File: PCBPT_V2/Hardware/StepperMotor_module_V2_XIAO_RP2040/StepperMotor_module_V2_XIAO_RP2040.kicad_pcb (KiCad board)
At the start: 2 copper layers, 43 x 43 mm, 32 parts, among them IC1 ICM-20649, J1 1660, J2 battery, J3 External Ctrl, J4 Conn_01x03_Pin, J5 SW, U1 MOUDLE-SEEEDUINO-XIAO, U2 MCP73831-2-OT, U3 AP2112K-3.3

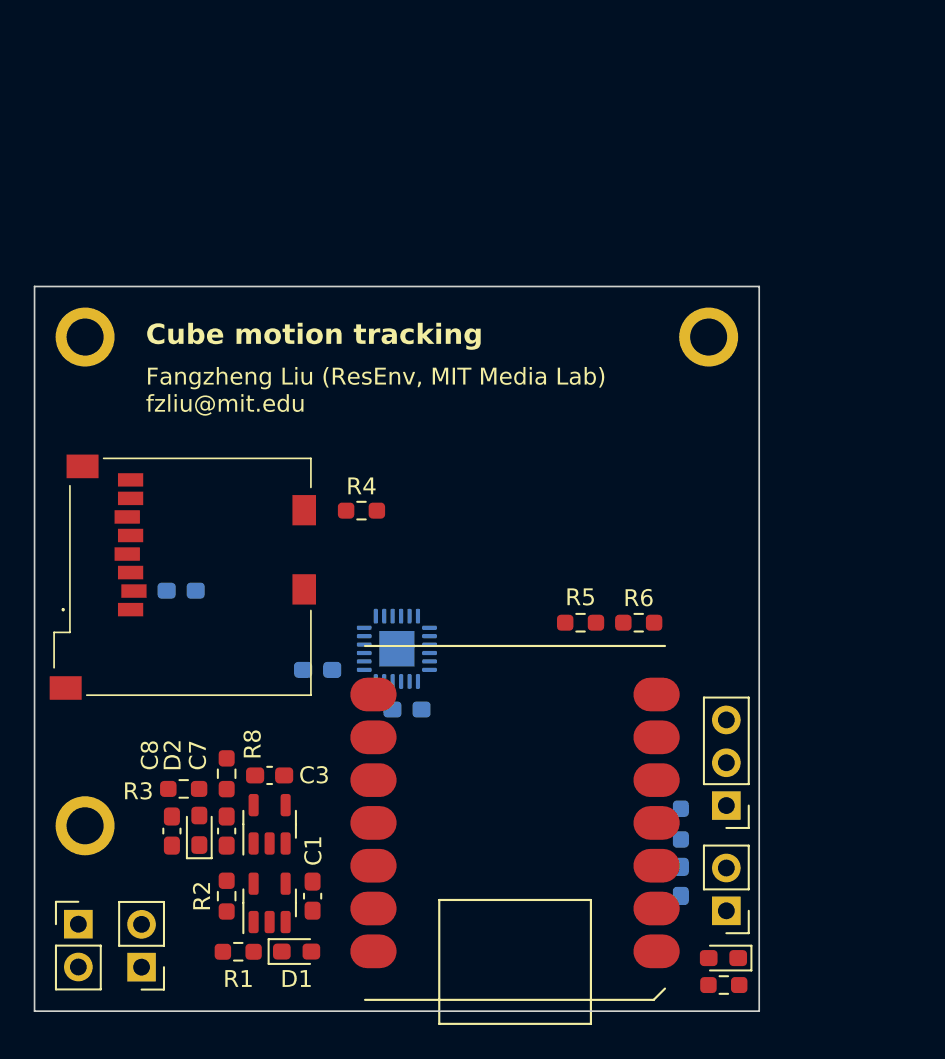
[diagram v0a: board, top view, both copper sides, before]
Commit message: udated by FZ
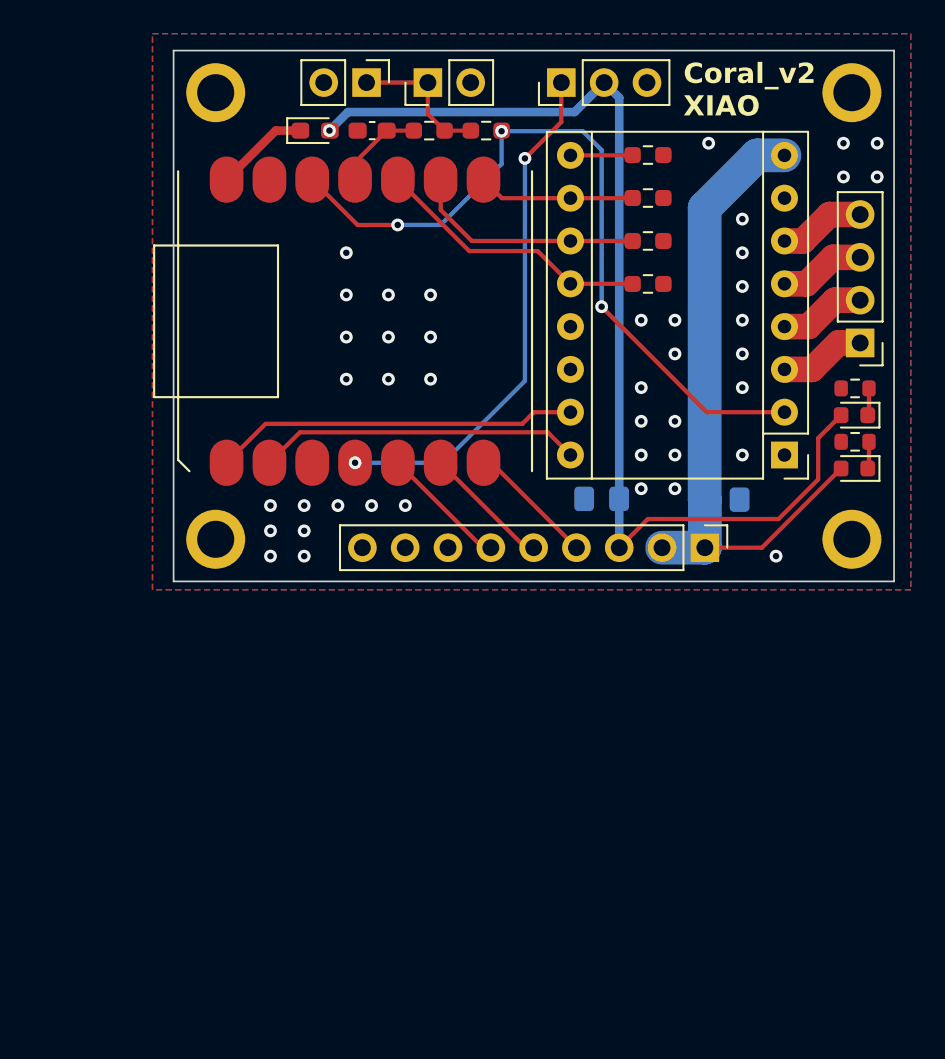
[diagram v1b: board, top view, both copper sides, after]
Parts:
- removed C4, C5, C6, C7: 0.1uF, Capacitor_SMD:C_0603_1608Metric_Pad1.08x0.95mm_HandSolder
- removed C8: 10uF, Capacitor_SMD:C_0603_1608Metric_Pad1.08x0.95mm_HandSolder
- removed C9: 0.01uF, Capacitor_SMD:C_0603_1608Metric_Pad1.08x0.95mm_HandSolder
- removed D3: Red, LED_SMD:LED_0603_1608Metric_Pad1.05x0.95mm_HandSolder
- removed IC1: ICM-20649, Package_DFN_QFN:HVQFN-24-1EP_4x4mm_P0.5mm_EP2.1x2.1mm
- removed J1: 1660, SamacSys_Parts:1660
- removed J2: battery, Connector_PinHeader_2.54mm:PinHeader_1x02_P2.54mm_Vertical
- removed R5, R6: 499K, Resistor_SMD:R_0603_1608Metric_Pad0.98x0.95mm_HandSolder
- removed R7, R9: 10K, Resistor_SMD:R_0603_1608Metric_Pad0.98x0.95mm_HandSolder
- removed U2: MCP73831-2-OT, Package_TO_SOT_SMD:SOT-23-5
- removed U3: AP2112K-3.3, Package_TO_SOT_SMD:SOT-23-5
- added A1: Pololu_Breakout_A4988, Module:Pololu_Breakout-16_15.2x20.3mm, F.Cu at (158.5, 82.0)
- added C2: 0.01uF, Capacitor_SMD:C_0603_1608Metric_Pad1.08x0.95mm_HandSolder, F.Cu at (134.0, 62.8)
- added D4: LED_Small_Filled, LED_SMD:LED_0603_1608Metric, F.Cu at (162.7, 82.8)
- added H4: M2, MountingHole:MountingHole_2.2mm_M2_ISO7380_Pad, F.Cu at (162.5, 60.5)
- added J6: Limit Switch, Connector_PinHeader_2.54mm:PinHeader_1x02_P2.54mm_Vertical, F.Cu at (133.7, 59.9)
- added J7: Limit Switch, Connector_PinHeader_2.54mm:PinHeader_1x02_P2.54mm_Vertical, F.Cu at (137.3, 59.9)
- added R10: 10k, Resistor_SMD:R_0603_1608Metric, F.Cu at (162.7, 81.2)
- added R11: 10K, Resistor_SMD:R_0603_1608Metric_Pad0.98x0.95mm_HandSolder, F.Cu at (140.8, 62.8)
- added R12: 100, Resistor_SMD:R_0603_1608Metric_Pad0.98x0.95mm_HandSolder, F.Cu at (137.4, 62.8)
- C1: footprint Capacitor_SMD:C_0603_1608Metric_Pad1.08x0.95mm_HandSolder -> Capacitor_SMD:C_0805_2012Metric_Pad1.18x1.45mm_HandSolder; moved to B.Cu
- C3: value 10uF -> 0.1uF; footprint Capacitor_SMD:C_0603_1608Metric_Pad1.08x0.95mm_HandSolder -> Capacitor_SMD:C_0805_2012Metric_Pad1.18x1.45mm_HandSolder; moved to B.Cu
- D1: value CHG -> LED_Small_Filled; footprint LED_SMD:LED_0603_1608Metric_Pad1.05x0.95mm_HandSolder -> LED_SMD:LED_0603_1608Metric
- J3: value External Ctrl -> Servo; footprint Connector_PinHeader_2.54mm:PinHeader_1x02_P2.54mm_Vertical -> Connector_PinHeader_2.54mm:PinHeader_1x03_P2.54mm_Vertical
- J4: value Conn_01x03_Pin -> Limit Switch; footprint Connector_PinHeader_2.54mm:PinHeader_1x03_P2.54mm_Vertical -> Connector_PinHeader_2.54mm:PinHeader_1x04_P2.54mm_Vertical
- J5: value SW -> Conn_01x09_Pin; footprint Connector_PinHeader_2.54mm:PinHeader_1x02_P2.54mm_Vertical -> Connector_PinHeader_2.54mm:PinHeader_1x09_P2.54mm_Vertical
- R1: value 1K -> 499K
- R2: value 1K -> 10K
- R3: value 1M -> 10K
- R4: value NC -> 10K
- R8: value 1M -> 10k; footprint Resistor_SMD:R_0603_1608Metric_Pad0.98x0.95mm_HandSolder -> Resistor_SMD:R_0603_1608Metric
- moved R1 53.2 mm to (150.4, 64.2)
- moved J3 50.1 mm to (145.3, 59.9), turned to 90 degrees
- moved R2 48.4 mm to (150.4, 66.8), turned to 0 degrees
- moved D1 45.9 mm to (162.7, 79.6), turned to 180 degrees
- moved R8 43.7 mm to (162.7, 78.0), turned to 180 degrees
- moved R3 42.6 mm to (150.4, 69.3)
- moved D2 42.1 mm to (130.7, 62.8), turned to 0 degrees
- moved J5 41.7 mm to (153.8, 87.5), turned to -90 degrees
- moved C1 33.8 mm to (154.8, 84.7), turned to 0 degrees
- moved J4 28.6 mm to (163.0, 75.3)
- moved C3 25.6 mm to (147.7, 84.6), turned to 180 degrees
- moved R4 21.7 mm to (150.4, 71.8)
- moved H1 18.7 mm to (124.8, 87.0)
- moved H2 16.4 mm to (124.8, 60.5)
- moved H3 14.7 mm to (162.5, 87.0)
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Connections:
- C1 pad 1: VBUS -> VPP
- C3 pad 1: +3V3 -> VCC
- D1 pad 2: VBUS -> VCC
- D2 pad 1: VBUS -> Net-(D2-K)
- D2 pad 2: +BATT -> VCC
- J3 pad 1: GND -> PWM_S
- J3 pad 2: /MCU-XIAO RP2040/EX_SIG -> VCC
- J4 pad 1: Net-(J4-Pin_1) -> 1B
- J4 pad 2: Net-(J4-Pin_2) -> 1A
- J4 pad 3: Net-(J4-Pin_3) -> 2A
- J5 pad 1: Net-(J2-Pin_2) -> VPP
- J5 pad 2: +BATT -> VPP
- R1 pad 1: Net-(D1-K) -> /A4988_Module/M_EN
- R1 pad 2: Net-(U2-STAT) -> GND
- R2 pad 1: Net-(U2-PROG) -> MS1
- R3 pad 1: GND -> MS2
- R3 pad 2: +BATT -> GND
- R4 pad 1: Net-(J1-CARD_DETECT_1) -> MS3
- R4 pad 2: +3V3 -> GND
- R8 pad 1: GND -> Net-(D1-K)
- R8 pad 2: +3V3 -> GND
- U1 pad 1: /MCU-XIAO RP2040/VBAT -> STEP
- U1 pad 10: MISO -> MS3
- U1 pad 11: MOSI -> LIMIT_SW_0
- U1 pad 12: unconnected-(U1-3V3-Pad12) -> +3V3
- U1 pad 14: VBUS -> Net-(D2-K)
- U1 pad 2: /MCU-XIAO RP2040/LED -> DIR
- U1 pad 3: /MCU-XIAO RP2040/EX_SIG -> unconnected-(U1-PA10_A2_D2-Pad3)
- U1 pad 4: Net-(J4-Pin_1) -> PWM_S
- U1 pad 5: Net-(J4-Pin_2) -> SDA
- U1 pad 6: Net-(J4-Pin_3) -> SCL
- U1 pad 7: IMU_CS -> GPIO
- U1 pad 8: SD_CS -> MS1
- U1 pad 9: SCK -> MS2
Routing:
- net VCC: track 0.00 -> 63.3 mm, vias 0 -> 1
- net +3V3: track 0.00 -> 44.9 mm, vias 0 -> 3
- net VPP: track 0.00 -> 38.8 mm
- net PWM_S: track 0.00 -> 30.7 mm, vias 0 -> 2
- net STEP: track 0.00 -> 21.6 mm
- net DIR: track 0.00 -> 19.2 mm
- net MS3: track 0.00 -> 16.5 mm
- net MS2: track 0.00 -> 13.9 mm
- net MS1: track 0.00 -> 9.31 mm
- net Net-(J6-Pin_1): track 0.00 -> 8.46 mm
- net SCL: track 0.00 -> 7.60 mm
- net SDA: track 0.00 -> 7.60 mm
- net GPIO: track 0.00 -> 7.60 mm
- net Net-(D2-K): track 0.00 -> 5.58 mm
- net LIMIT_SW_0: track 0.00 -> 5.30 mm
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- added copper zone on B.Cu, net GND
- added copper zone on F.Cu, net GND
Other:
- board size 43 x 43 mm -> 42.8 x 31.5 mm
- board text added: "Coral_v2 XIAO"
- board text removed: "Cube motion tracking"
- board text removed: "Fangzheng Liu (ResEnv, MIT Media Lab) fzliu@mit.edu"
